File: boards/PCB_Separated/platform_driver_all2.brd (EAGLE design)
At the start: 18 parts, among them IC1 L293D

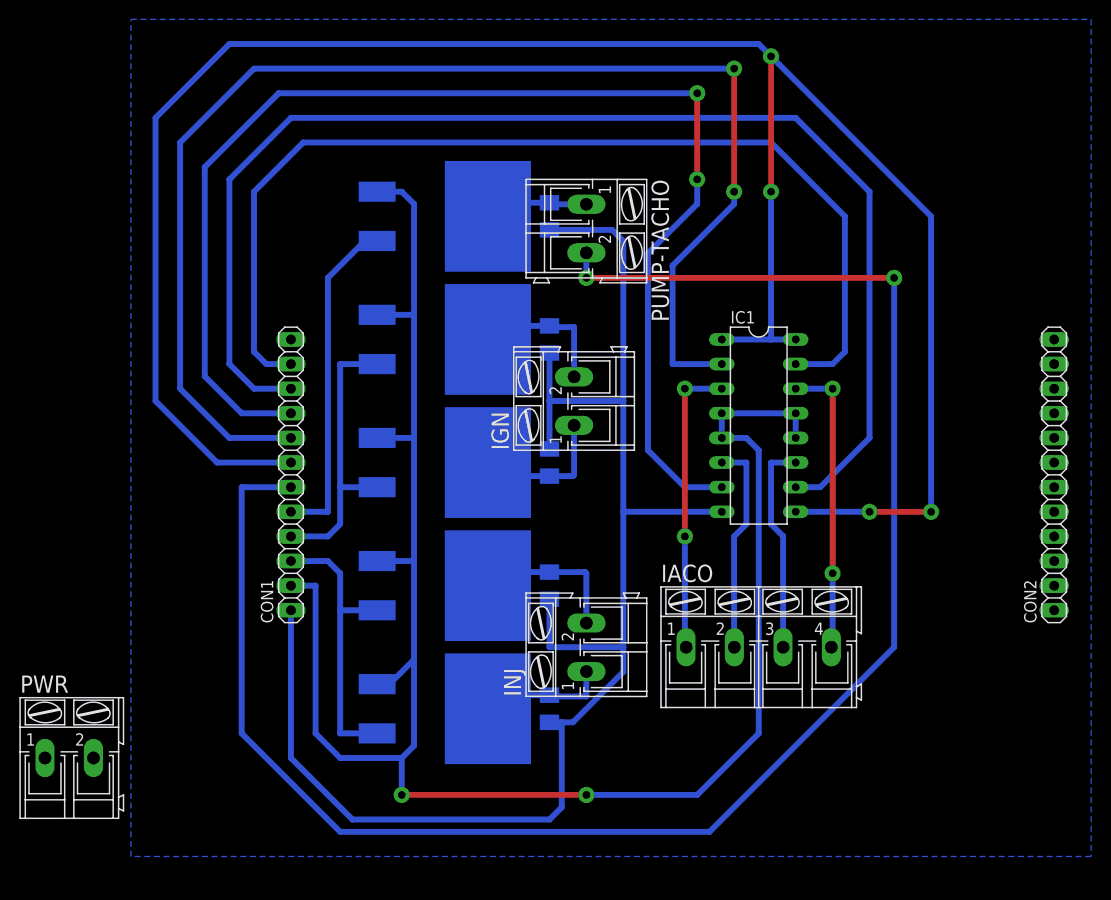
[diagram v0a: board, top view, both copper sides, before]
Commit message: revisi driver
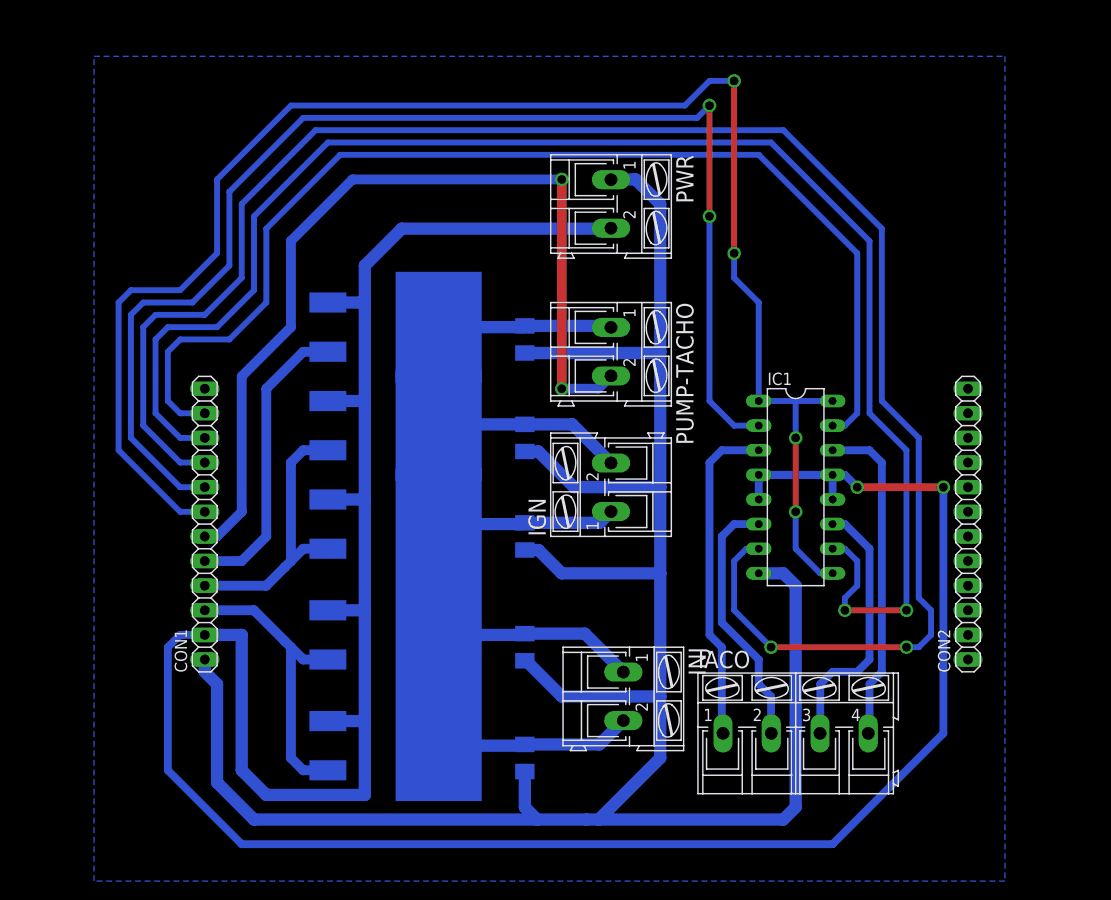
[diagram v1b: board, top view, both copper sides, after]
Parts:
- moved PWR 79.9 mm to (50.8, 67.3), turned to 270 degrees
- moved R-INJ2 18.0 mm to (41.9, 10.2)
- moved FET-INJ2 17.3 mm to (30.5, 11.4)
- moved R-PUMP 13.0 mm to (41.9, 53.3)
- moved PUMP-TACHO 13.0 mm to (50.8, 52.1)
- moved FET-PUMP 12.5 mm to (30.5, 54.6)
- moved R-IGN2 10.5 mm to (41.9, 43.2)
- moved CON1 10.2 mm to (8.89, 34.3)
- moved CON2 10.2 mm to (87.6, 34.3)
- moved FET-IGN2 10.2 mm to (30.5, 44.5)
- moved IGN 9.67 mm to (50.8, 38.1)
- moved IACO 9.67 mm to (69.8, 12.7)
- moved FET-INJ1 9.16 mm to (30.5, 22.9)
- moved FET-IGN1 8.13 mm to (30.5, 34.3)
- moved R-IGN1 8.03 mm to (41.9, 33.0), turned to 270 degrees
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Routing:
- net GND: track 195.5 -> 294.8 mm
- net TACHOO: track 182.3 -> 92.7 mm
- net V12: track 157.7 -> 239.9 mm
- net IAC2: track 134.1 -> 186.0 mm
- net VCC2: track 217.6 -> 166.0 mm
- net IAC3: track 133.4 -> 159.2 mm, vias 0 -> 2
- net IAC4: track 106.6 -> 117.2 mm
- net INJ1O: track 13.4 -> 20.7 mm
- net PUMPO: track 10.8 -> 17.9 mm
- net IAC3O: track 22.1 -> 27.5 mm
- net IAC1: track 137.4 -> 132.1 mm
- net IGN2O: track 14.7 -> 19.5 mm
- net IAC2O: track 22.1 -> 26.8 mm
- net PUMP: track 34.6 -> 30.6 mm
- net IGN1O: track 14.6 -> 18.3 mm
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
